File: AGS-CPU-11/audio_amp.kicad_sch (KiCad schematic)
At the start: 43 parts, among them U3 AGB-AMP, U9 RN4986

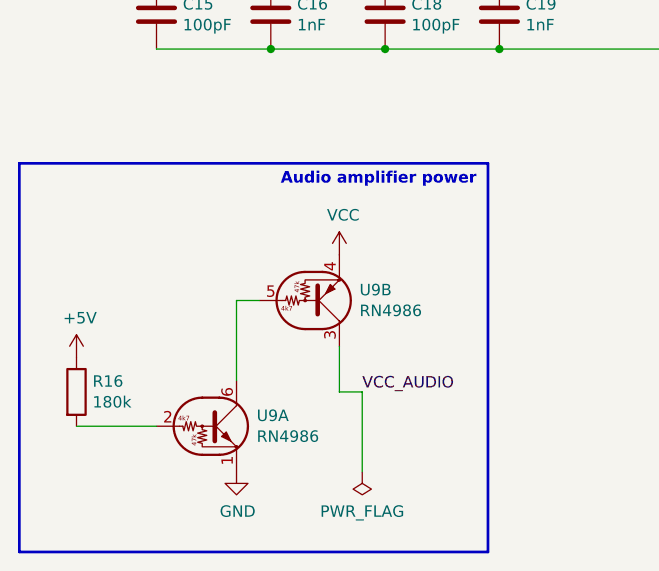
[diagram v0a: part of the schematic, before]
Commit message: Update to latest KiCad
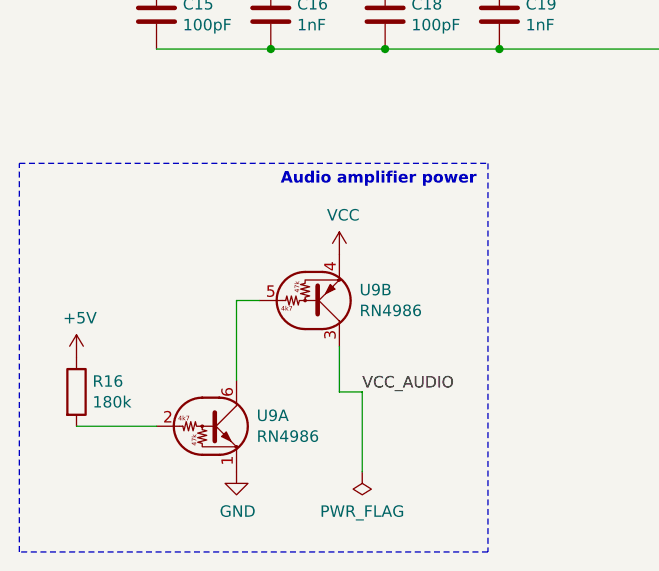
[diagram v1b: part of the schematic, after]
